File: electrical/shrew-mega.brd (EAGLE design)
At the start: 18 x 15 mm, 21 parts, among them U1 DRV8244SQRYJRQ1, U2 DRV8244SQRYJRQ1, X1 PIN-1X-BIG, X2 PIN-1X-BIG, X3 PIN-1X-BIG, X4 PIN-1X-BIG, X5 PIN-1X-BIG, X6 PIN-1X-BIG

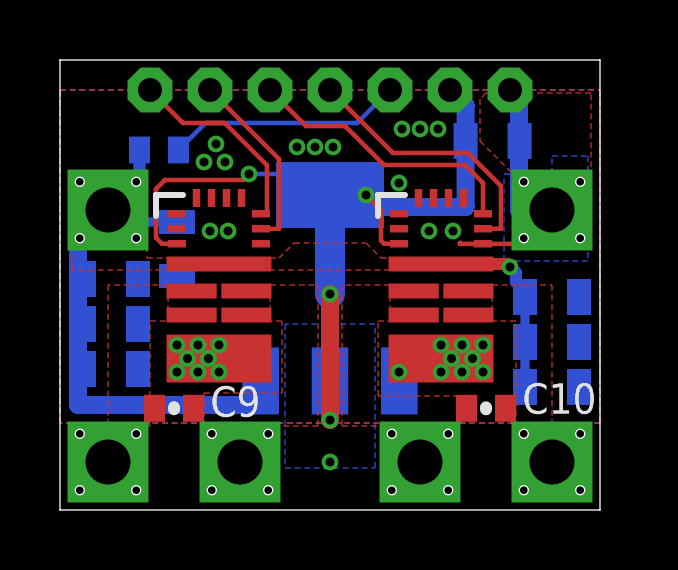
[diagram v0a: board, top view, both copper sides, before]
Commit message: more mfg files
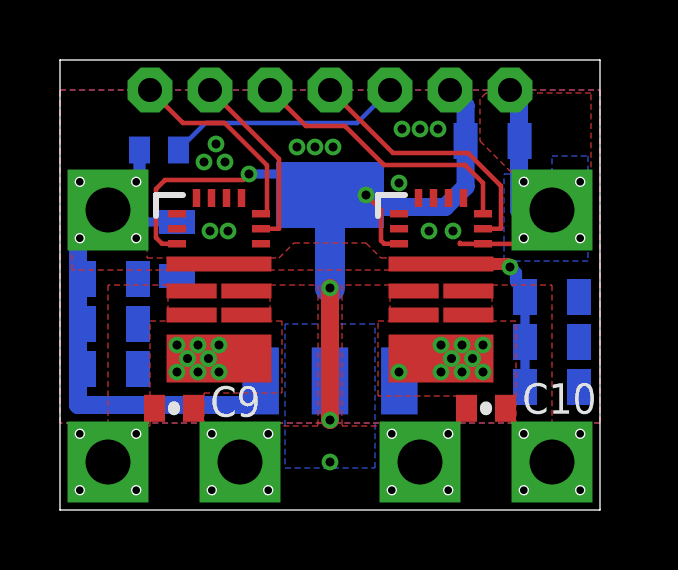
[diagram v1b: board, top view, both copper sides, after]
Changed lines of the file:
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@@
 <layer number="19" name="Unrouted" color="6" fill="1" visible="yes" active="yes"/>
 <layer number="20" name="Dimension" color="15" fill="1" visible="yes" active="yes"/>
-<layer number="21" name="tPlace" color="7" fill="1" visible="no" active="yes"/>
-<layer number="22" name="bPlace" color="7" fill="1" visible="no" active="yes"/>
+<layer number="21" name="tPlace" color="7" fill="1" visible="yes" active="yes"/>
+<layer number="22" name="bPlace" color="7" fill="1" visible="yes" active="yes"/>
 <layer number="23" name="tOrigins" color="15" fill="1" visible="no" active="yes"/>
 <layer number="24" name="bOrigins" color="15" fill="1" visible="no" active="yes"/>
@@
 <layer number="39" name="tKeepout" color="4" fill="11" visible="no" active="yes"/>
 <layer number="40" name="bKeepout" color="1" fill="11" visible="no" active="yes"/>
-<layer number="41" name="tRestrict" color="4" fill="10" visible="yes" active="yes"/>
-<layer number="42" name="bRestrict" color="1" fill="10" visible="yes" active="yes"/>
+<layer number="41" name="tRestrict" color="4" fill="10" visible="no" active="yes"/>
+<layer number="42" name="bRestrict" color="1" fill="10" visible="no" active="yes"/>
 <layer number="43" name="vRestrict" color="2" fill="10" visible="no" active="yes"/>
 <layer number="44" name="Drills" color="7" fill="1" visible="no" active="yes"/>
@@
 <wire x1="18" y1="15" x2="0" y2="15" width="0" layer="20"/>
 <wire x1="0" y1="15" x2="0" y2="0" width="0" layer="20"/>
-<rectangle x1="1.5" y1="3.3" x2="5.7" y2="4.8" layer="30"/>
 <wire x1="2.14" y1="7.88" x2="2.14" y2="4.48" width="0" layer="42"/>
 <wire x1="2.14" y1="4.48" x2="2.13" y2="4.48" width="0" layer="42"/>
@@
 <polygon width="0" layer="29" spacing="0.254">
 <vertex x="3.6" y="7.6"/>
-<vertex x="1.5" y="7.6"/>
-<vertex x="1.5" y="2.7"/>
+<vertex x="1.6" y="7.6"/>
+<vertex x="1.6" y="2.7"/>
 <vertex x="3" y="2.7"/>
 <vertex x="3" y="6.3"/>
@@
 <polygon width="0" layer="29" spacing="0.254">
 <vertex x="7" y="7.6"/>
-<vertex x="8.3" y="7.6"/>
-<vertex x="8.3" y="6.6"/>
-<vertex x="8.3" y="2.9"/>
+<vertex x="8.5" y="7.6"/>
+<vertex x="8.5" y="2.9"/>
 <vertex x="6.3" y="2.9"/>
 <vertex x="6.3" y="3.9"/>
-<vertex x="6.5" y="3.9"/>
 <vertex x="7.4" y="3.9"/>
 <vertex x="7.4" y="6.3"/>
@@
 <vertex x="11.8" y="3.8"/>
 <vertex x="11.8" y="2.8"/>
-<vertex x="9.7" y="2.8"/>
-<vertex x="9.7" y="7.6"/>
+<vertex x="9.5" y="2.8"/>
+<vertex x="9.5" y="7.6"/>
 </polygon>
 <polygon width="0" layer="29" spacing="0.254">
@@
 <vertex x="14.5" y="6.3"/>
 </polygon>
-<wire x1="0.2" y1="14.4" x2="18" y2="14.4" width="0" layer="41"/>
+<wire x1="0.1" y1="14" x2="17.9" y2="14" width="0" layer="41"/>
 <wire x1="18" y1="14.4" x2="0.2" y2="14.4" width="0" layer="42"/>
 </plain>
@@
 <wire x1="10.2" y1="11.2" x2="10.2" y2="10.5" width="0.6" layer="16"/>
 <via x="9" y="3" extent="1-16" drill="0.3" shape="octagon"/>
-<wire x1="9" y1="3" x2="9" y2="7.2" width="0.6" layer="1"/>
-<via x="9" y="7.2" extent="1-16" drill="0.3" shape="octagon"/>
-<wire x1="9" y1="7.2" x2="9" y2="10.499" width="1" layer="16"/>
+<wire x1="9" y1="3" x2="9" y2="7.4" width="0.6" layer="1"/>
+<via x="9" y="7.4" extent="1-16" drill="0.3" shape="octagon"/>
+<wire x1="9" y1="7.4" x2="9" y2="10.499" width="1" layer="16"/>
 <wire x1="9" y1="4.3012" x2="9" y2="3" width="0.6" layer="16"/>
 <wire x1="13" y1="14" x2="13.52" y2="13.48" width="0.6" layer="16"/>
 <wire x1="13.52" y1="13.48" x2="13.52" y2="12.3" width="0.6" layer="16"/>
-<wire x1="13.52" y1="12.3" x2="13.52" y2="10.1" width="0.6" layer="16"/>
-<wire x1="13.52" y1="10.1" x2="10.2" y2="10.1" width="0.6" layer="16"/>
+<wire x1="13.52" y1="12.3" x2="13.52" y2="10.78" width="0.6" layer="16"/>
+<wire x1="13.52" y1="10.78" x2="12.84" y2="10.1" width="0.6" layer="16"/>
+<wire x1="12.84" y1="10.1" x2="10.2" y2="10.1" width="0.6" layer="16"/>
 <wire x1="10.2" y1="10.1" x2="10.2" y2="10.5" width="0.6" layer="16"/>
 <wire x1="3.2" y1="10.7" x2="3.5" y2="11" width="0.1524" layer="1"/>
@@
 <wire x1="6.1" y1="11" x2="6.3" y2="11.2" width="0.1524" layer="1"/>
 <via x="6.3" y="11.2" extent="1-16" drill="0.3" shape="octagon"/>
-<wire x1="6.3" y1="11.2" x2="8.299" y2="11.2" width="0.1524" layer="16"/>
+<wire x1="6.3" y1="11.2" x2="8.299" y2="11.2" width="0.3048" layer="16"/>
 <wire x1="8.299" y1="11.2" x2="9" y2="10.499" width="0.1524" layer="16"/>
 </signal>
